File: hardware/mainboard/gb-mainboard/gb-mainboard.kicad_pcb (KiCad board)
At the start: 2 copper layers, 77.4 x 81 mm, 0 parts

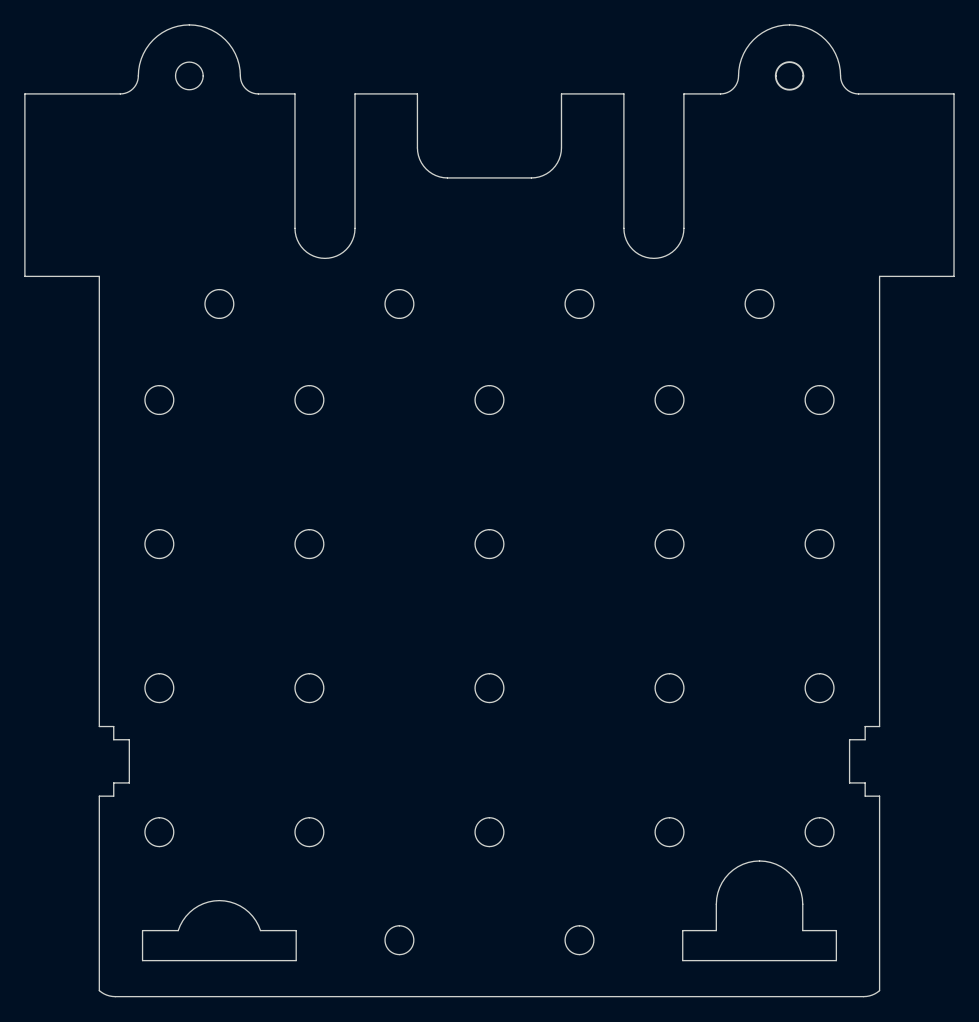
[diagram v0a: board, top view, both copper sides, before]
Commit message: .
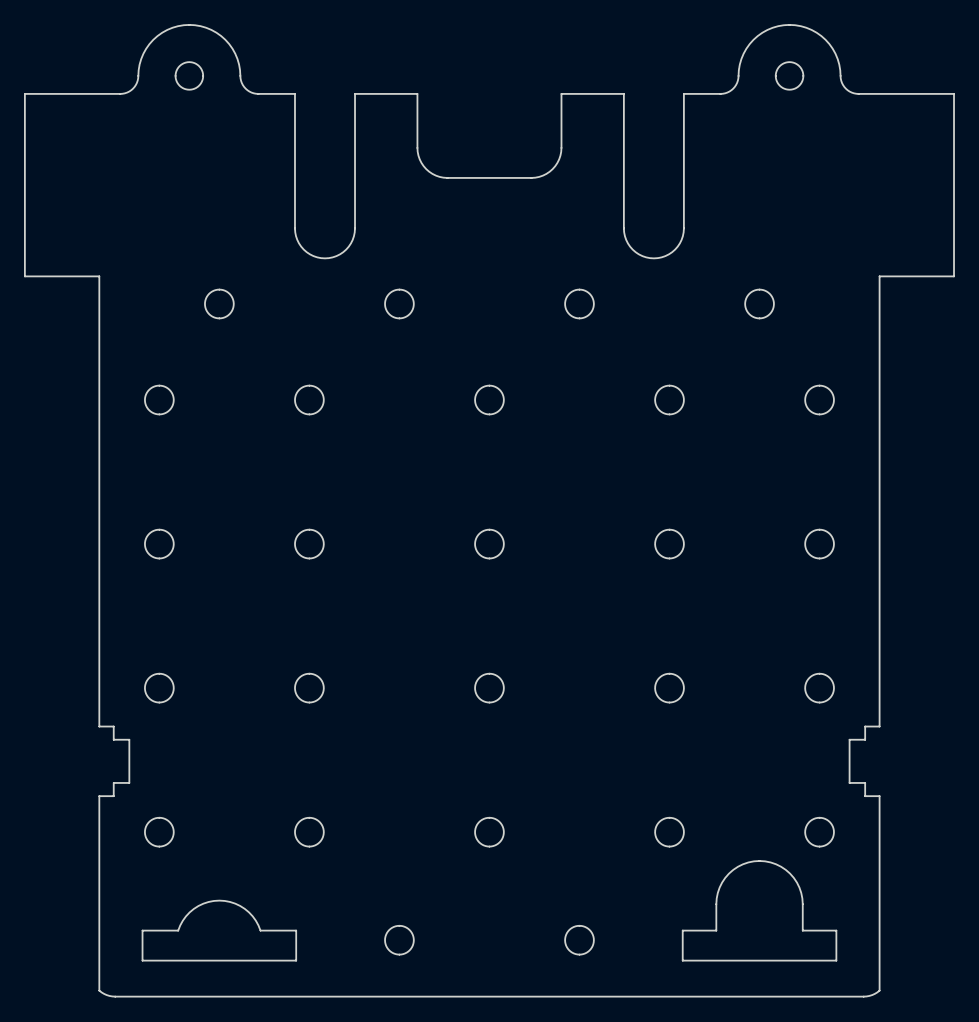
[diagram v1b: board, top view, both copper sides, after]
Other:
- net class Default: trace_width 0.25 -> 0.15
